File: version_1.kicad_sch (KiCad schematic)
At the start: 27 parts, among them U1 Pico, U10 74AHC595, U12 C967633

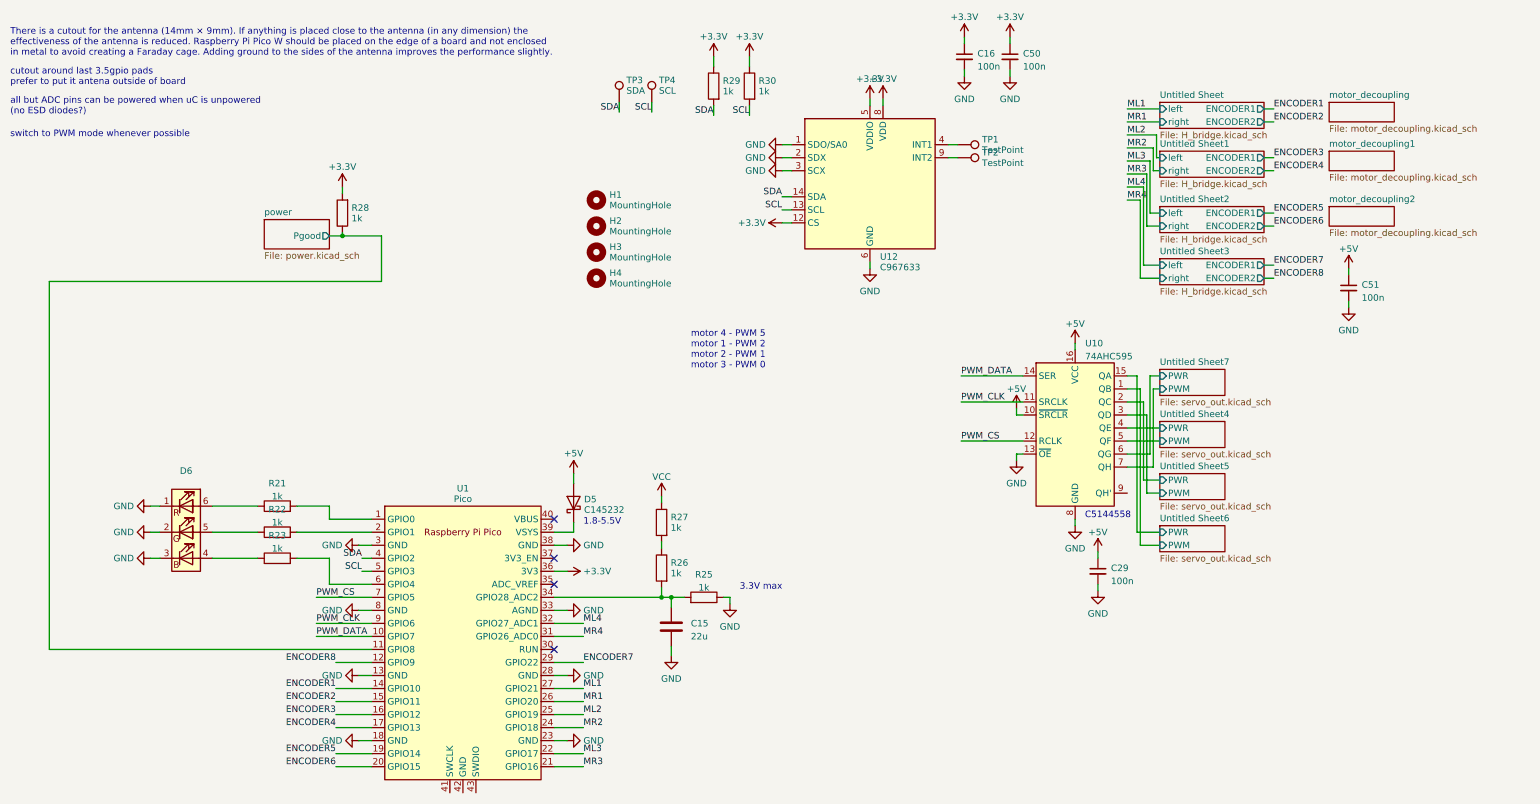
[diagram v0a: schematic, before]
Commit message: added moany componaets
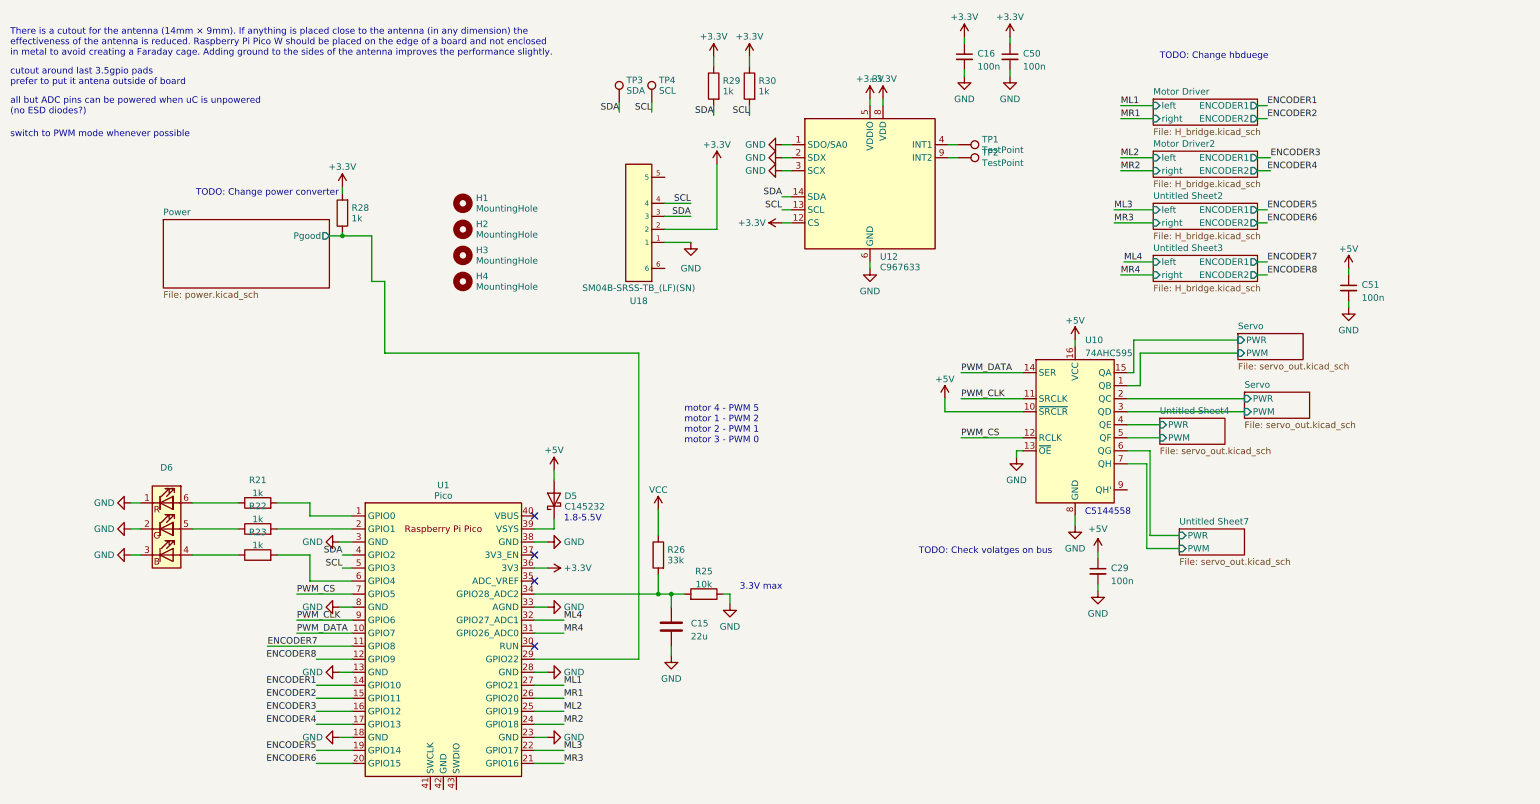
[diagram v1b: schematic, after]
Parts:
- removed R27: 1k, Resistor_SMD:R_0603_1608Metric_Pad0.98x0.95mm_HandSolder, symbol Device:R
- added U18: SM04B-SRSS-TB_(LF)(SN), footprint:CONN-SMD_4P-P1.00_SM04B-SRSS-TB-LF-SN, symbol SM04B-SRSS-TB_(LF)(SN):SM04B-SRSS-TB_(LF)(SN)
- R25: value 1k -> 10k
- R26: value 1k -> 33k
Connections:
- net Untitled Sheet5/PWM is gone; now on net Servo/PWM: U10.3 (QD)
- net Untitled Sheet5/PWR is gone; now on net Servo/PWR: U10.2 (QC)
- net +3.3V: now also U18.2
- net ENCODER7: now also U1.11 (GPIO8); no longer U1.29 (GPIO22)
- net GND: now also U18.1
- net SCL: now also U18.4
- net SDA: now also U18.3
- net Servo/PWM: no longer U10.1 (QB)
- net Servo/PWR: no longer U10.15 (QA)
- net VCC: now also R26.1
- net Power/Pgood: now also U1.29 (GPIO22); no longer U1.11 (GPIO8)
- new net Servo/PWM: U10.1 (QB)
- new net Servo/PWR: U10.15 (QA)
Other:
- sheet Untitled Sheet renamed Motor Driver
- sheet Untitled Sheet1 renamed Motor Driver2
- sheet Untitled Sheet6 renamed Servo
- sheet power renamed Power
- removed sheet Untitled Sheet5
- removed sheet motor_decoupling
- removed sheet motor_decoupling1
- removed sheet motor_decoupling2
- note added: "TODO: Change hbduege"
- note added: "TODO: Change power converter"
- note added: "TODO: Check volatges on bus"
- moved on the sheet: D5, D6, H1, H2, H3, H4, R21, R22, R23, R25, R26, U1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
